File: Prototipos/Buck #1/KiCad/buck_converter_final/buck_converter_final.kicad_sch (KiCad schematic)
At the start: 25 parts, among them J1 Conn_01x03_Pin, J2 Screw_Terminal_01x02, J3 Screw_Terminal_01x02, Q1 IRF9540NPBF, Q3 NPN

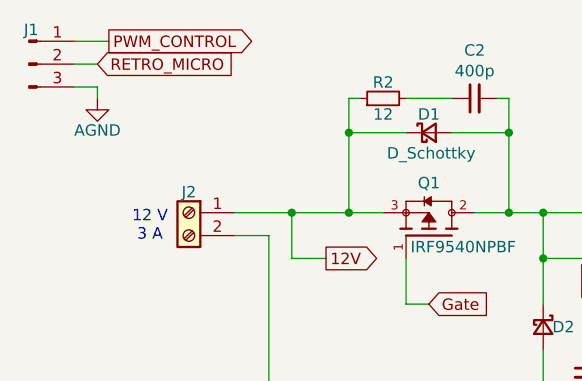
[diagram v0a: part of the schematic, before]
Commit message: Primera versión PCB final Buck
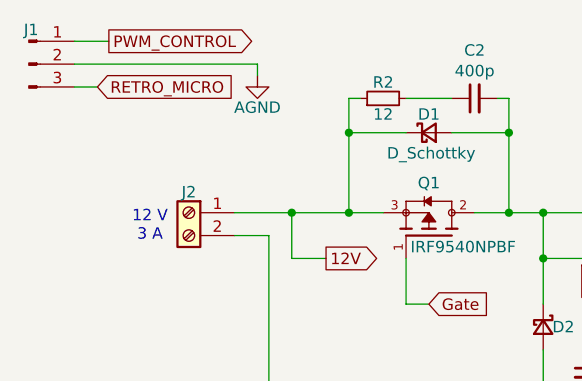
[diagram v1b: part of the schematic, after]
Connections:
- net AGND: now also J1.2 (Pin_2); no longer J1.3 (Pin_3)
- net RETRO_MICRO: now also J1.3 (Pin_3); no longer J1.2 (Pin_2)
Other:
- company: (none) -> Alesandria - Cignetti - Galliano
- title: (none) -> PCB final Convertidor Buck
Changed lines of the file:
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@@
 	(generator_version "9.0")
 	(paper "A4")
+	(title_block
+		(title "PCB final Convertidor Buck")
+		(company "Alesandria - Cignetti - Galliano")
+	)
 	(rectangle
 		(start 130.81 85.09)
@@
 	(wire
 		(pts
+			(xy 81.28 38.1) (xy 101.6 38.1)
+		)
+		(stroke
+			(width 0)
+			(type default)
+		)
+	)
+	(wire
+		(pts
 			(xy 102.87 81.28) (xy 133.35 81.28)
 		)
@@
 	(wire
 		(pts
-			(xy 81.28 38.1) (xy 83.82 38.1)
-		)
-		(stroke
-			(width 0)
-			(type default)
-		)
-	)
-	(wire
-		(pts
 			(xy 133.35 81.28) (xy 149.86 81.28)
 		)
@@
 	(wire
 		(pts
-			(xy 81.28 40.64) (xy 83.82 40.64)
-		)
-		(stroke
-			(width 0)
-			(type default)
-		)
-	)
-	(wire
-		(pts
 			(xy 138.43 64.77) (xy 138.43 69.85)
 		)
@@
 	(wire
 		(pts
+			(xy 83.82 40.64) (xy 81.28 40.64)
+		)
+		(stroke
+			(width 0)
+			(type default)
+		)
+	)
+	(wire
+		(pts
 			(xy 118.11 41.91) (xy 123.19 41.91)
 		)
@@
 	(wire
 		(pts
-			(xy 83.82 40.64) (xy 83.82 41.91)
-		)
-		(stroke
-			(width 0)
-			(type default)
-		)
-	)
-	(wire
-		(pts
 			(xy 156.21 87.63) (xy 156.21 90.17)
 		)
@@
 		(pts
 			(xy 181.61 96.52) (xy 181.61 95.25)
+		)
+		(stroke
+			(width 0)
+			(type default)
+		)
+	)
+	(wire
+		(pts
+			(xy 101.6 38.1) (xy 101.6 39.37)
 		)
 		(stroke
@@
 	(global_label "RETRO_MICRO"
 		(shape input)
-		(at 83.82 38.1 0)
+		(at 83.82 40.64 0)
 		(fields_autoplaced yes)
 		(effects
@@
 		)
 		(property "Intersheetrefs" "${INTERSHEET_REFS}"
-			(at 99.6866 38.1 0)
+			(at 99.6866 40.64 0)
 			(effects
 				(font
@@
 	(symbol
 		(lib_id "power:GND")
-		(at 83.82 41.91 0)
+		(at 101.6 39.37 0)
 		(unit 1)
 		(exclude_from_sim no)
@@
 		(dnp no)
 		(property "Reference" "#PWR01"
-			(at 83.82 48.26 0)
+			(at 101.6 45.72 0)
 			(effects
 				(font
@@
 		)
 		(property "Value" "AGND"
-			(at 83.82 45.466 0)
+			(at 101.6 42.926 0)
 			(effects
 				(font
@@
 		)
 		(property "Footprint" ""
-			(at 83.82 41.91 0)
+			(at 101.6 39.37 0)
 			(effects
 				(font
@@
 		)
 		(property "Datasheet" ""
-			(at 83.82 41.91 0)
+			(at 101.6 39.37 0)
 			(effects
 				(font
@@
 		)
 		(property "Description" "Power symbol creates a global label with name \"GND\" , ground"
-			(at 83.82 41.91 0)
-			(effects
-				(font
+			(at 101.6 39.37 0)
+			(effects
+				(font
